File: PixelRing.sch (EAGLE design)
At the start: 40 parts, among them Q1 CMA-4544PF-W, SW1 SPST_TACT-KMR2, SW2 SPST_TACT-KMR2, U1 MAX4466EXK+T

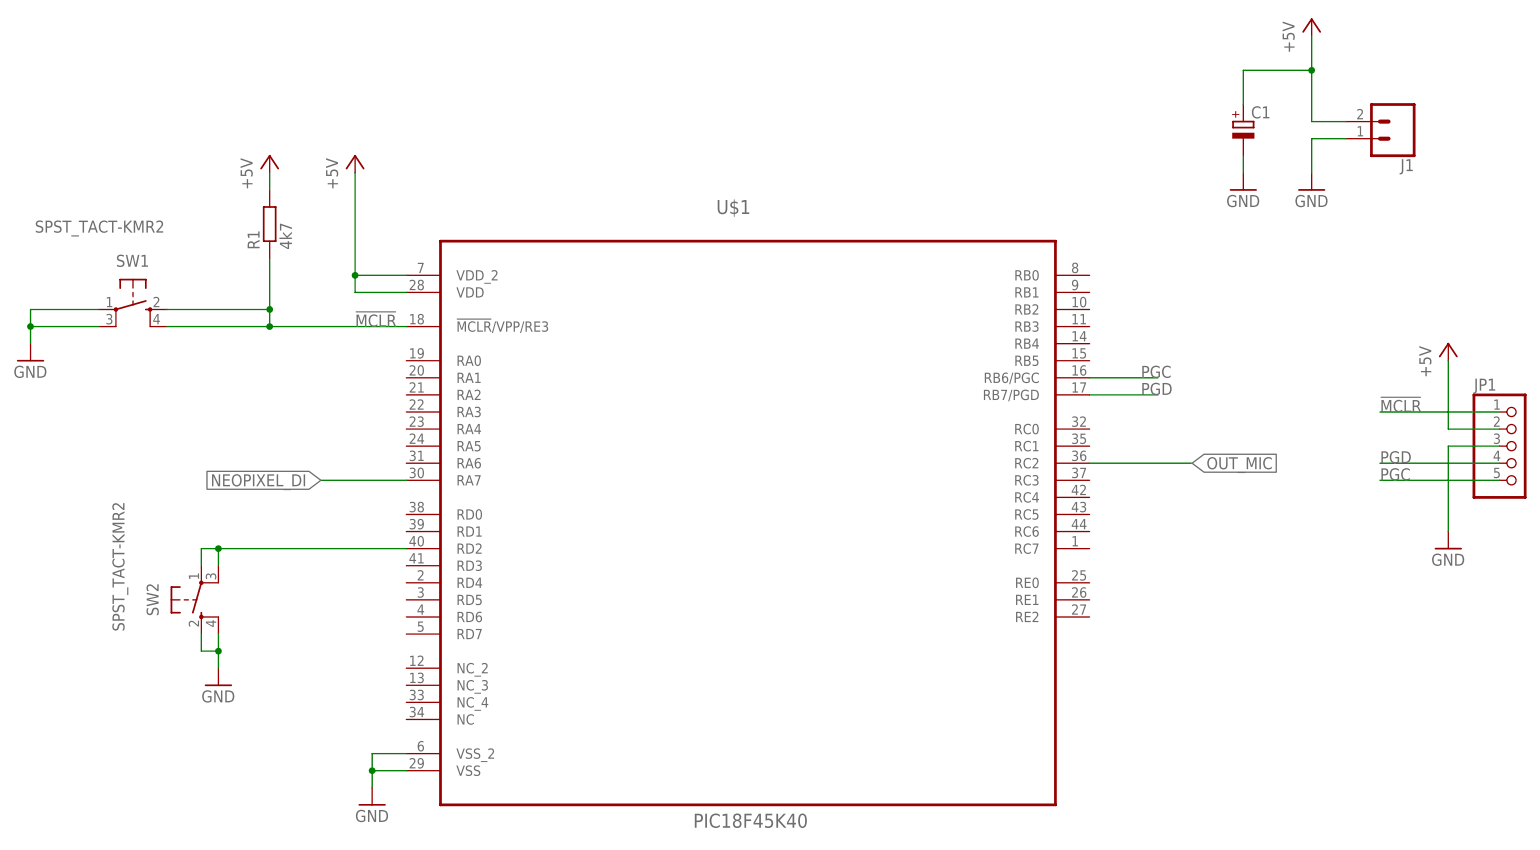
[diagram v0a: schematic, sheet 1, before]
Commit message: Add files via upload
Changed micro
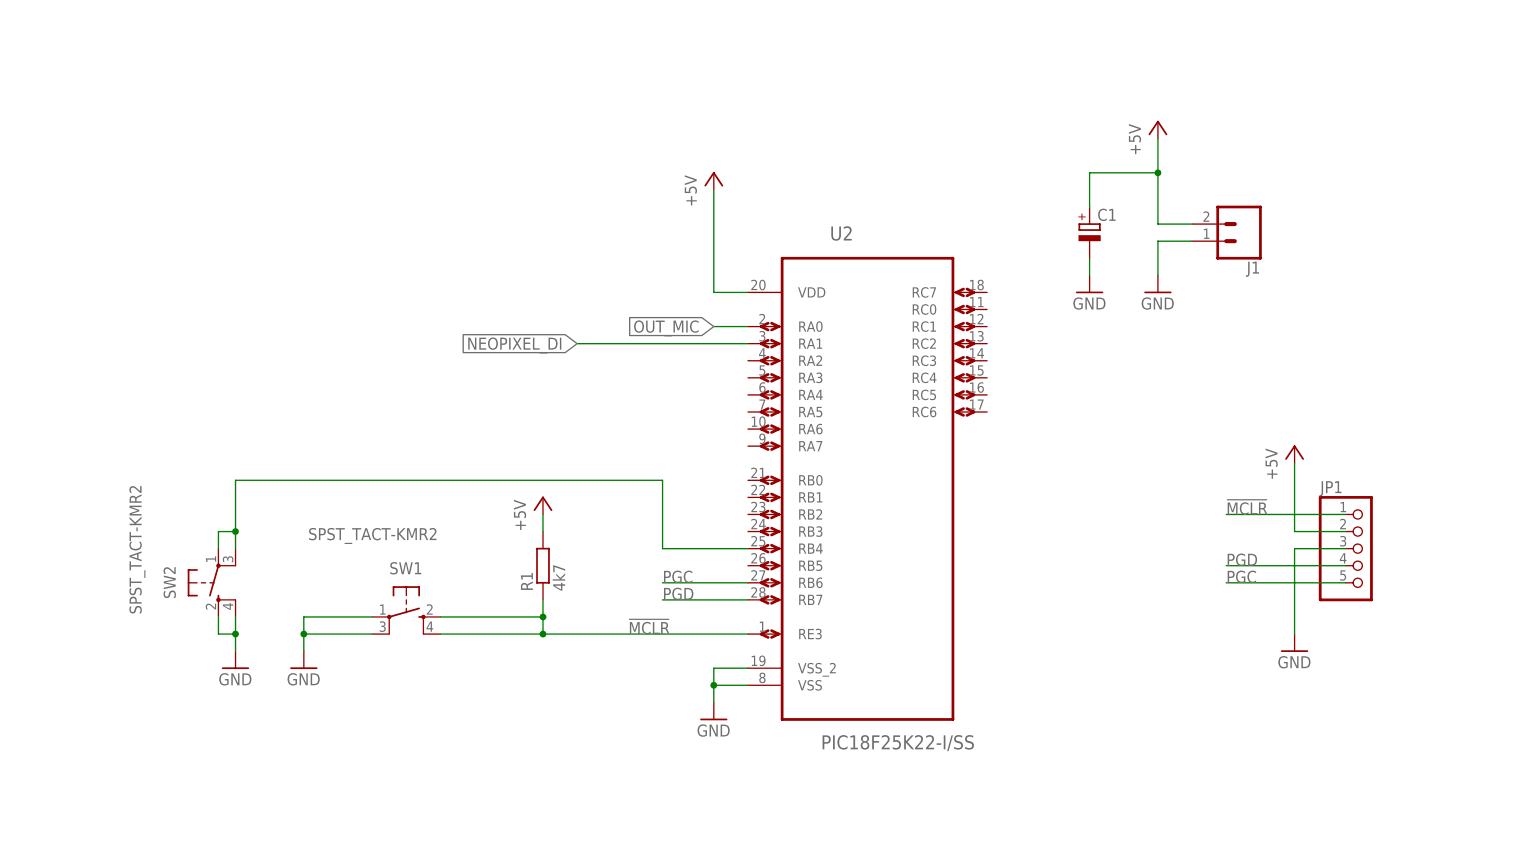
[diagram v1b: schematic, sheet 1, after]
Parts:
- removed U$1: PIC18F45K40, 0_Lib_IRSEEM:PIC18F45K40
- added U2: PIC18F25K22-I/SS, 0_Lib_IRSEEM:PIC18F25K22-I/SS
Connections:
- removed net N$15: SW2.P, SW2.P1, U$1.RD2
- new net N$19: SW2.P, SW2.P1, U2.RB4
- net !MCLR: now also U2.RE3; no longer U$1.!MCLR!/VPP/RE3
- net +5V: now also U2.VDD; no longer U$1.VDD, U$1.VDD_2
- net GND: now also U2.VSS, U2.VSS_2; no longer U$1.VSS, U$1.VSS_2
- net NEOPIXEL_DI: now also U2.RA1; no longer U$1.RA7
- net OUT_MIC: now also U2.RA0; no longer U$1.RC2
- net PGC: now also U2.RB6; no longer U$1.RB6/PGC
- net PGD: now also U2.RB7; no longer U$1.RB7/PGD
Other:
- moved on the sheet: C1, J1, JP1, R1, SW1, SW2
